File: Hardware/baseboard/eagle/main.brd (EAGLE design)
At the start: 119.5 x 96 mm, 173 parts, among them X1 JST-4POS-2X4POS, X1.2 TACH/LAP, X2 ATLAS-LTC, X2.1 MOTOR, X2.2 VRAILS+, X2.3 5V+SoC, X4 SYSTEWI, X5 15244441

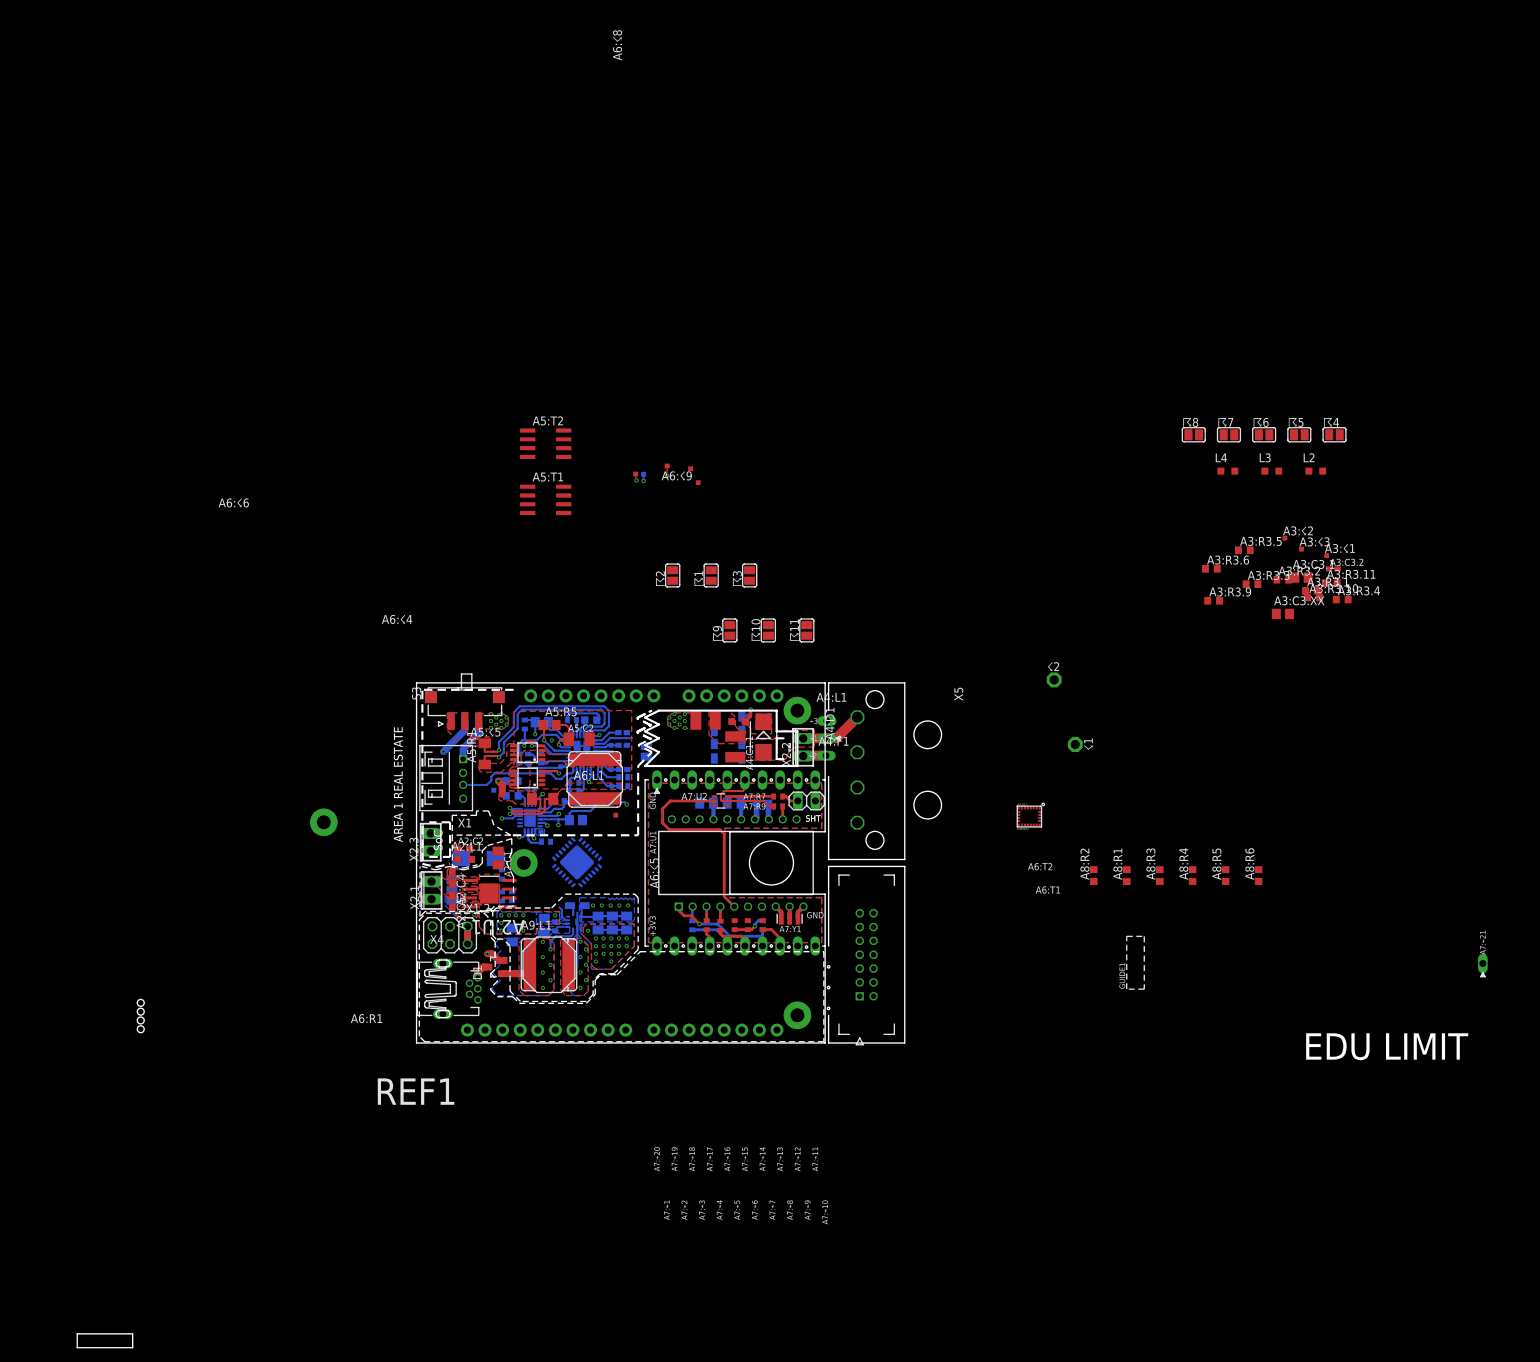
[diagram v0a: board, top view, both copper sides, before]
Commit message: wip baseboard quicksave  + nothing of high importance to see here  + just saving before merging LSM9DS1 from old design    to save time
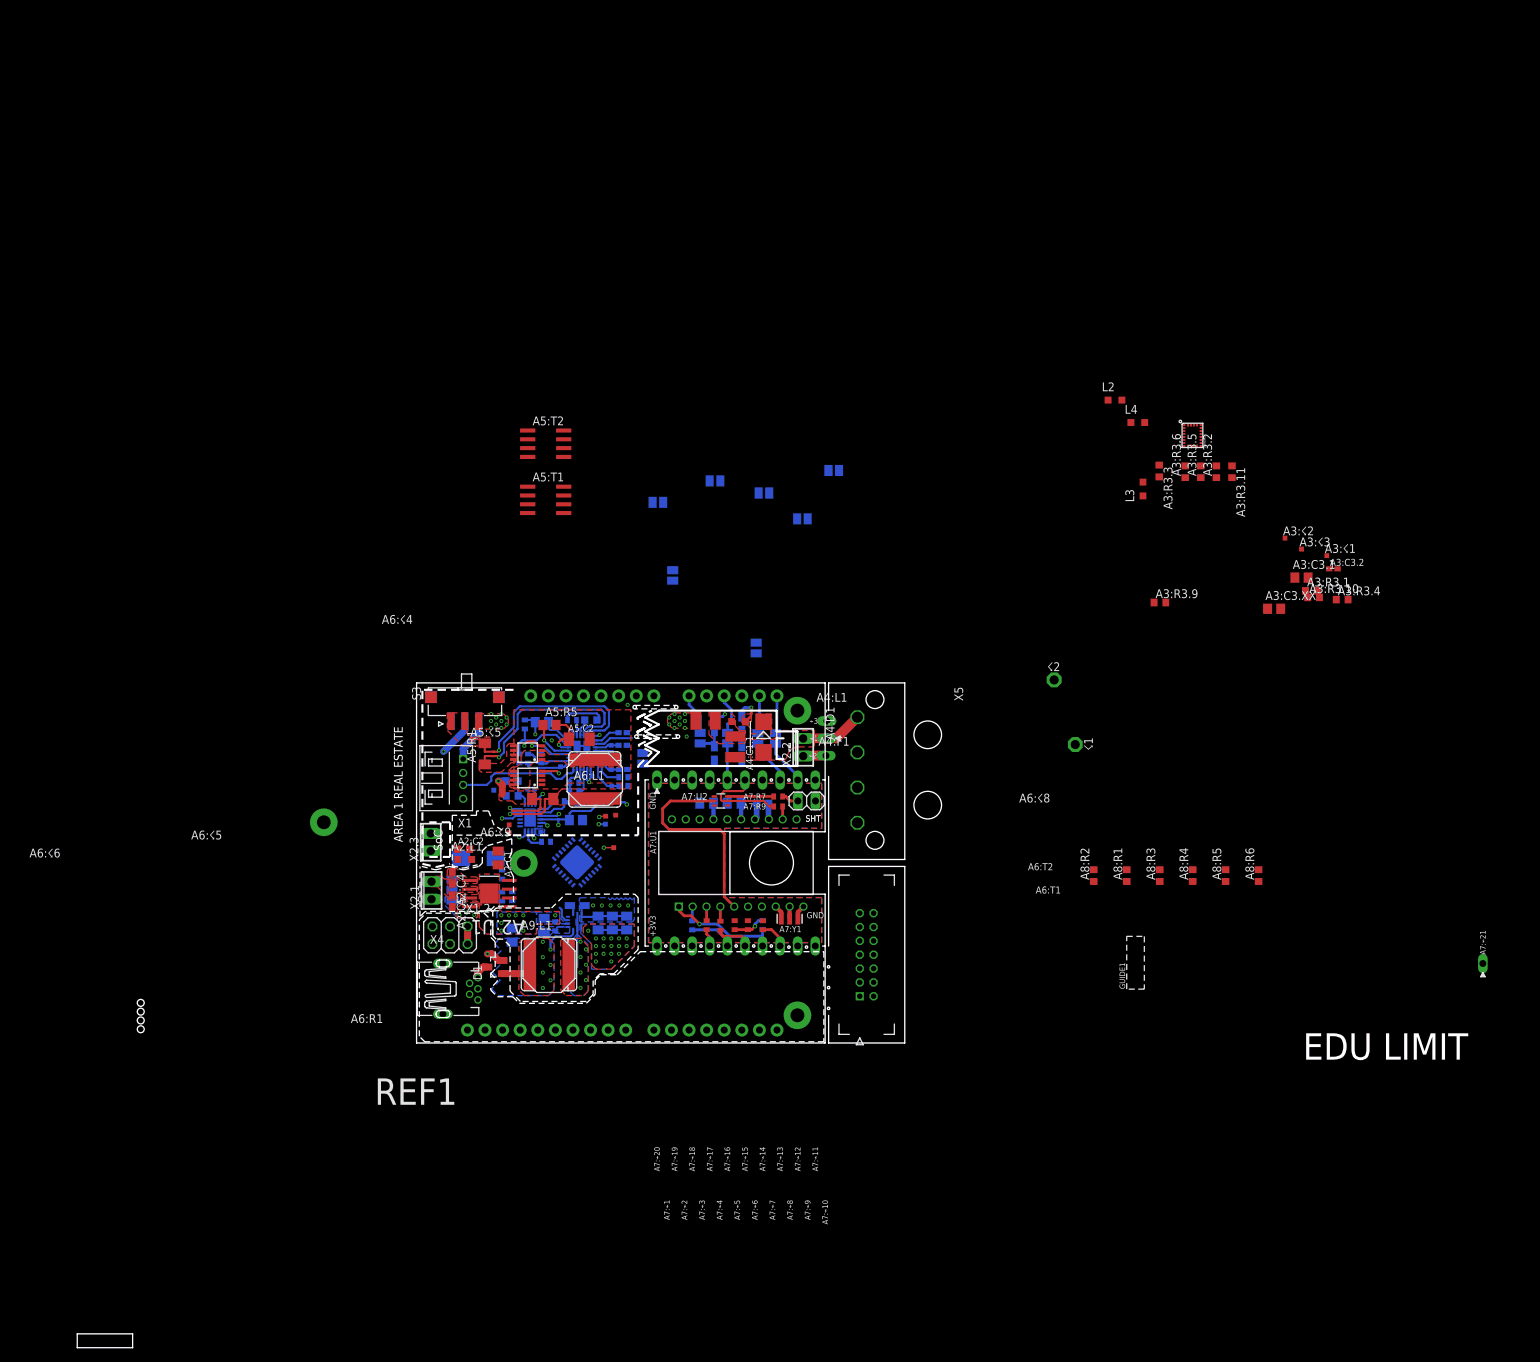
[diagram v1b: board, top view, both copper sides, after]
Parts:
- moved ☈4 98.2 mm to (39.8, 81.1), flipped to the bottom
- moved ☈8 69.5 mm to (48.1, 84.2), flipped to the bottom
- moved ☈6 67.8 mm to (60.7, 78.7), flipped to the bottom
- moved ☈7 67.7 mm to (55.2, 82.4), flipped to the bottom
- moved ☈5 67.4 mm to (65.2, 85.7), flipped to the bottom
- moved A3:U3.1 60.7 mm to (118.3, 89.2), turned to 90 degrees
- moved A6:☇9 57.7 mm to (18.4, 34.5)
- moved A6:☇6 57.5 mm to (18.4, 33.4)
- moved A6:☇5 55.7 mm to (33.5, 31.2), turned to 180 degrees
- moved A6:☇1 50.8 mm to (32.3, 34.6), turned to 270 degrees
- moved A6:☇8 49.6 mm to (32.3, 35.7), turned to 0 degrees
- moved L2 30.8 mm to (105.9, 95.8)
- moved ☈3 23.7 mm to (49.9, 47.0), flipped to the bottom
- moved ☈1 23.5 mm to (46.0, 47.0), flipped to the bottom
- moved A3:R3.11 21.5 mm to (122.8, 85.5), turned to 270 degrees
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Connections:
- removed net A4:COM.RRX: A4:R1.1, A4:R2.2
- removed net A4:MON.VPWR: A4:R3.1, A4:R4.2
- removed net COM.RRX: XA1.IO.7
- removed net MON.VPWR: ☈1.1
- new net TOP.MVPRW: A4:R3.1, A4:R4.2, ☈1.1
- new net TOP.RRX: A4:R1.1, A4:R2.2, XA1.IO.7
- net +3V3: no longer ☈9.1
- net +5V: no longer ☈3.1
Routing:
- net CORE.ADCX: track 0.00 -> 6.58 mm
- net CORE.ADCY: track 0.00 -> 6.58 mm
- net N$15: track 0.00 -> 6.01 mm
- net N$11: track 0.00 -> 6.01 mm
- net N$29: track 0.00 -> 5.47 mm
- net N$30: track 0.00 -> 5.45 mm
- net +5V: track 13.0 -> 18.2 mm
- net TOP.MVPRW: track 0.00 -> 4.62 mm
- net A4:N$1: track 4.19 -> 6.46 mm
- net TOP.RRX: track 0.00 -> 2.18 mm
- net +18V: track 0.55 -> 2.21 mm, vias 0 -> 1
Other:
- outline, holes or cut-outs redrawn
- board text added: ">verify footprint and import rather"
- board text added: "ERROR"
- board text added: "Y AM I DOING THIS AGAIN?"
- board text removed: ">geht ned"
- board text removed: "LX"
